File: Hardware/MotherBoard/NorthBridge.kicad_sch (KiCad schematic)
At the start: 4 parts, among them U6 74HC148, U7 74HC574, U8 ATF22V10B

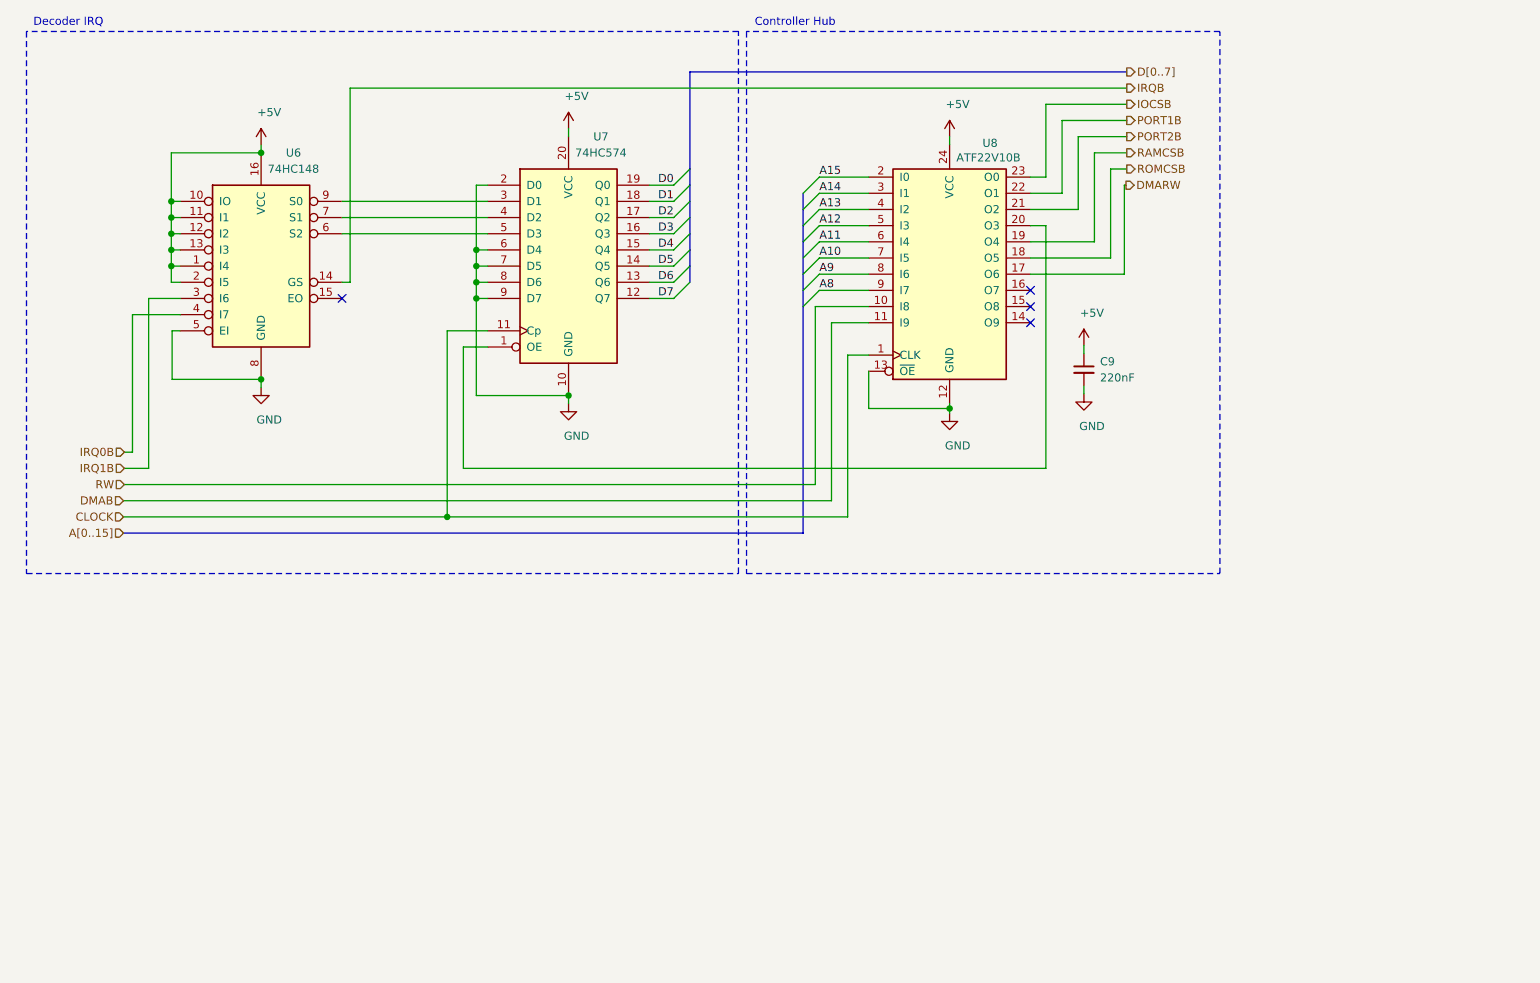
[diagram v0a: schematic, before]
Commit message: New motherboard version
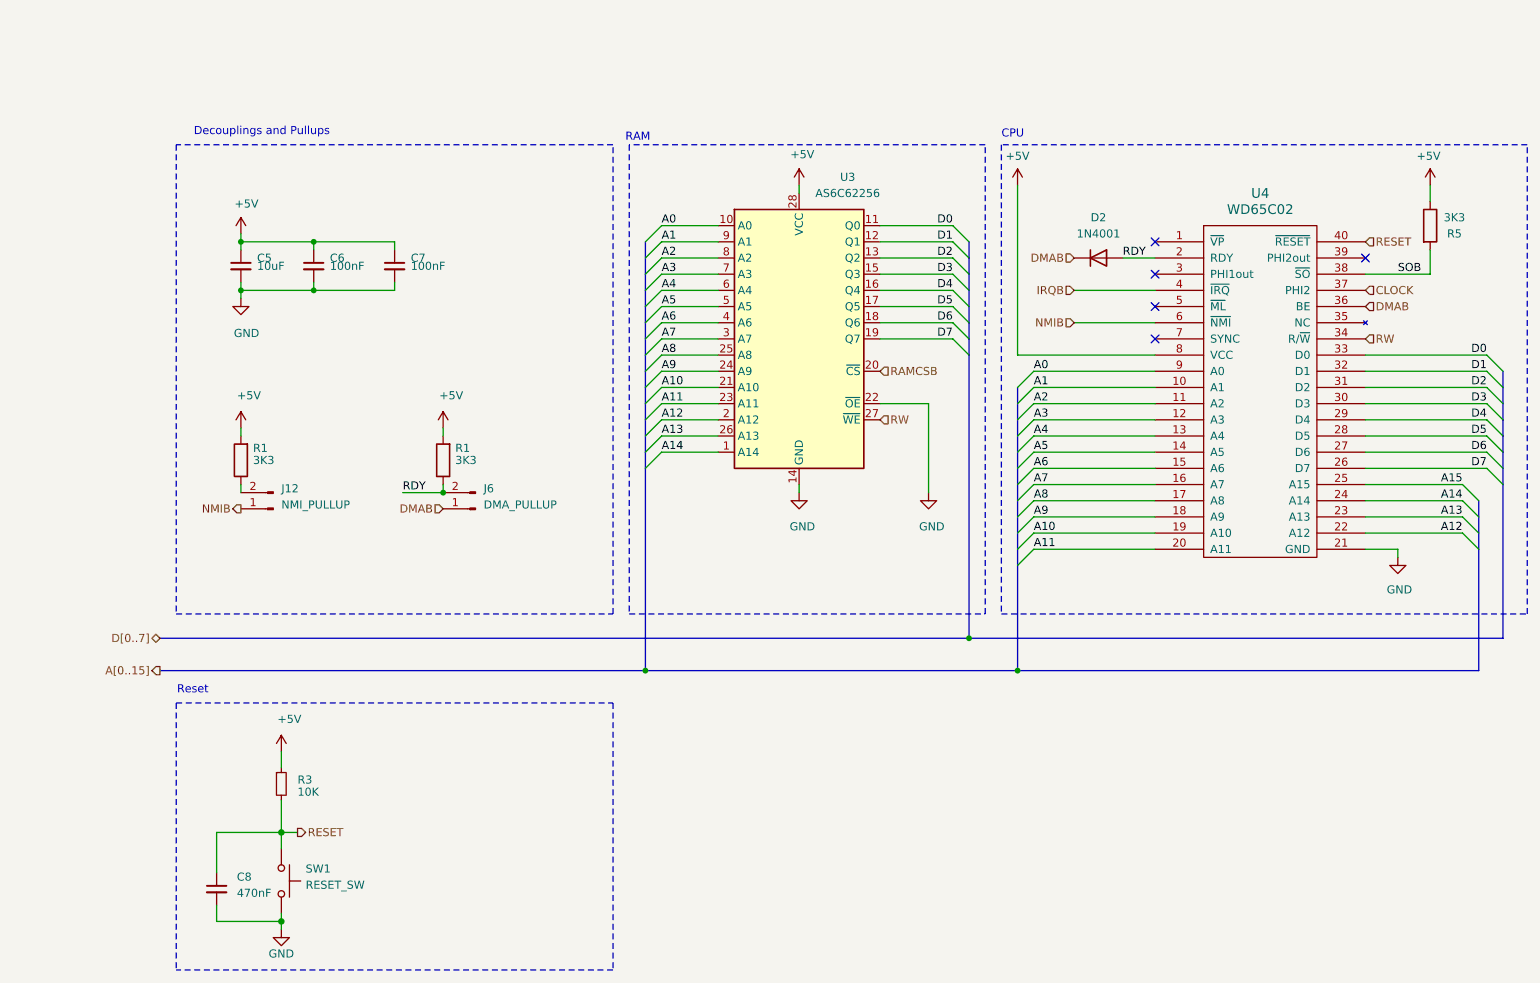
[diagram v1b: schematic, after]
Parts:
- removed C9: 220nF, Capacitor_THT:C_Disc_D5.0mm_W2.5mm_P5.00mm, symbol Device:C_Small
- removed U6: 74HC148, Package_DIP:DIP-16_W7.62mm, symbol 74xx:74LS148
- removed U7: 74HC574, Package_DIP:DIP-20_W7.62mm, symbol 74xx:74HCT574
- removed U8: ATF22V10B, Package_DIP:DIP-24_W7.62mm, symbol Logic_Programmable:PAL20RS10
- added C5: 10uF, Capacitor_THT:C_Radial_D5.0mm_H11.0mm_P2.00mm, symbol Device:C_Small
- added C6, C7: 100nF, Capacitor_THT:C_Disc_D5.0mm_W2.5mm_P2.50mm, symbol Device:C_Small
- added C8: 470nF, Capacitor_THT:C_Disc_D5.0mm_W2.5mm_P5.00mm, symbol Device:C_Small
- added D2: 1N4001, Diode_THT:D_DO-41_SOD81_P10.16mm_Horizontal, symbol Diode:1N4001
- added J12: NMI_PULLUP, Connector_PinHeader_2.54mm:PinHeader_1x02_P2.54mm_Vertical, symbol Connector:Conn_01x02_Pin
- added J6: DMA_PULLUP, Connector_PinHeader_2.54mm:PinHeader_1x02_P2.54mm_Vertical, symbol Connector:Conn_01x02_Pin
- added R1 (x2), R5: 3K3, Resistor_THT:R_Axial_DIN0207_L6.3mm_D2.5mm_P10.16mm_Horizontal, symbol Device:R
- added R3: 10K, Resistor_THT:R_Axial_DIN0207_L6.3mm_D2.5mm_P10.16mm_Horizontal, symbol Device:R_Small
- added SW1: RESET_SW, Button_Switch_THT:SW_Tactile_SPST_Angled_PTS645Vx83-2LFS, symbol Switch:SW_Push
- added U3: AS6C62256, Package_DIP:DIP-28_W15.24mm, symbol Memory_RAM:HM62256BLP
- added U4: WD65C02, Package_DIP:DIP-40_W15.24mm, symbol 65xx:WD65C02
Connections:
- net +5V: now also C5.1, C6.1, C7.1, R1.2, R1.2, R3.1, R5.1, U3.28 (VCC), U4.8 (VCC)
- net A10: now also U3.21 (A10), U4.19 (A10)
- net A11: now also U3.23 (A11), U4.20 (A11)
- net A12: now also U3.2 (A12), U4.22 (A12)
- net A13: now also U3.26 (A13), U4.23 (A13)
- net A14: now also U3.1 (A14), U4.24 (A14)
- net A15: now also U4.25 (A15)
- net A8: now also U3.25 (A8), U4.17 (A8)
- net A9: now also U3.24 (A9), U4.18 (A9)
- net CLOCK: now also U4.37 (PHI2)
- net D0: now also U3.11 (Q0), U4.33 (D0)
- net D1: now also U3.12 (Q1), U4.32 (D1)
- net D2: now also U3.13 (Q2), U4.31 (D2)
- net D3: now also U3.15 (Q3), U4.30 (D3)
- net D4: now also U3.16 (Q4), U4.29 (D4)
- net D5: now also U3.17 (Q5), U4.28 (D5)
- net D6: now also U3.18 (Q6), U4.27 (D6)
- net D7: now also U3.19 (Q7), U4.26 (D7)
- net DMAB: now also D2.1 (K), J6.1 (Pin_1), U4.36 (BE)
- net GND: now also C5.2, C6.2, C7.2, C8.2, SW1.2, U3.14 (GND), U3.22 (~{OE}), U4.21 (GND)
- net IRQB: now also U4.4 (~{IRQ})
- net RAMCSB: now also U3.20 (~{CS})
- net RW: now also U3.27 (~{WE}), U4.34 (R/~{W})
- new net: J12.2 (Pin_2), R1.1
- new net A0: U3.10 (A0), U4.9 (A0)
- new net A1: U3.9 (A1), U4.10 (A1)
- new net A2: U3.8 (A2), U4.11 (A2)
- new net A3: U3.7 (A3), U4.12 (A3)
- new net A4: U3.6 (A4), U4.13 (A4)
- new net A5: U3.5 (A5), U4.14 (A5)
- new net A6: U3.4 (A6), U4.15 (A6)
- new net A7: U3.3 (A7), U4.16 (A7)
- new net NMIB: J12.1 (Pin_1), U4.6 (~{NMI})
- new net RDY: D2.2 (A), J6.2 (Pin_2), R1.1, U4.2 (RDY)
- new net RESET: C8.1, R3.2, SW1.1, U4.40 (~{RESET})
- new net SOB: R5.2, U4.38 (~{SO})
- no-connect marks 4 -> 5
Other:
- note added: "CPU"
- note added: "Decouplings and Pullups"
- note added: "RAM"
- note added: "Reset"
- note removed: "Controller Hub"
- note removed: "Decoder IRQ"
